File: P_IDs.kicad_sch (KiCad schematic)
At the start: 0 parts

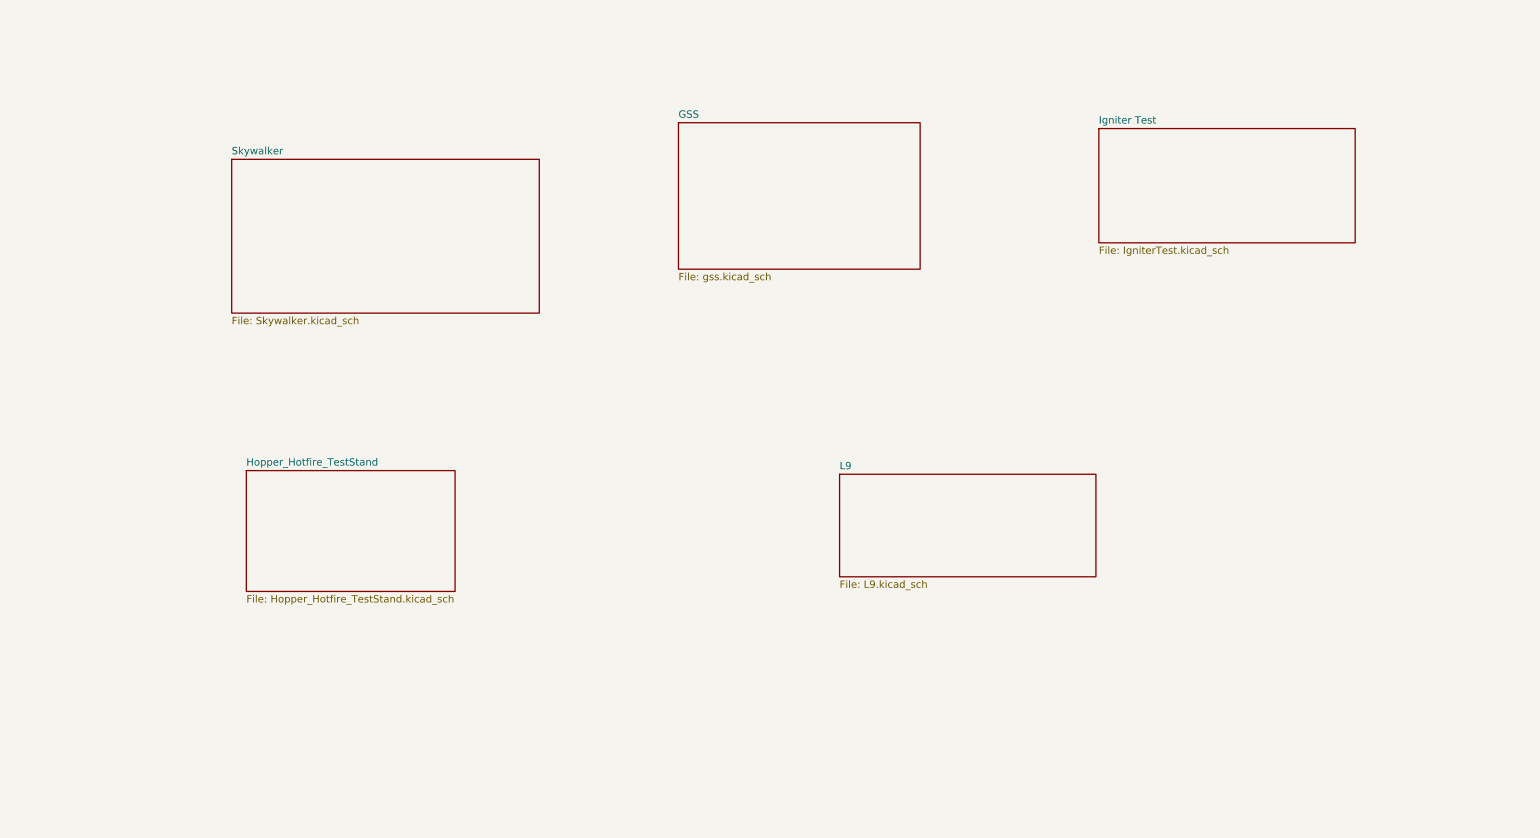
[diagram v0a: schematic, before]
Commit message: igniter+hotfire
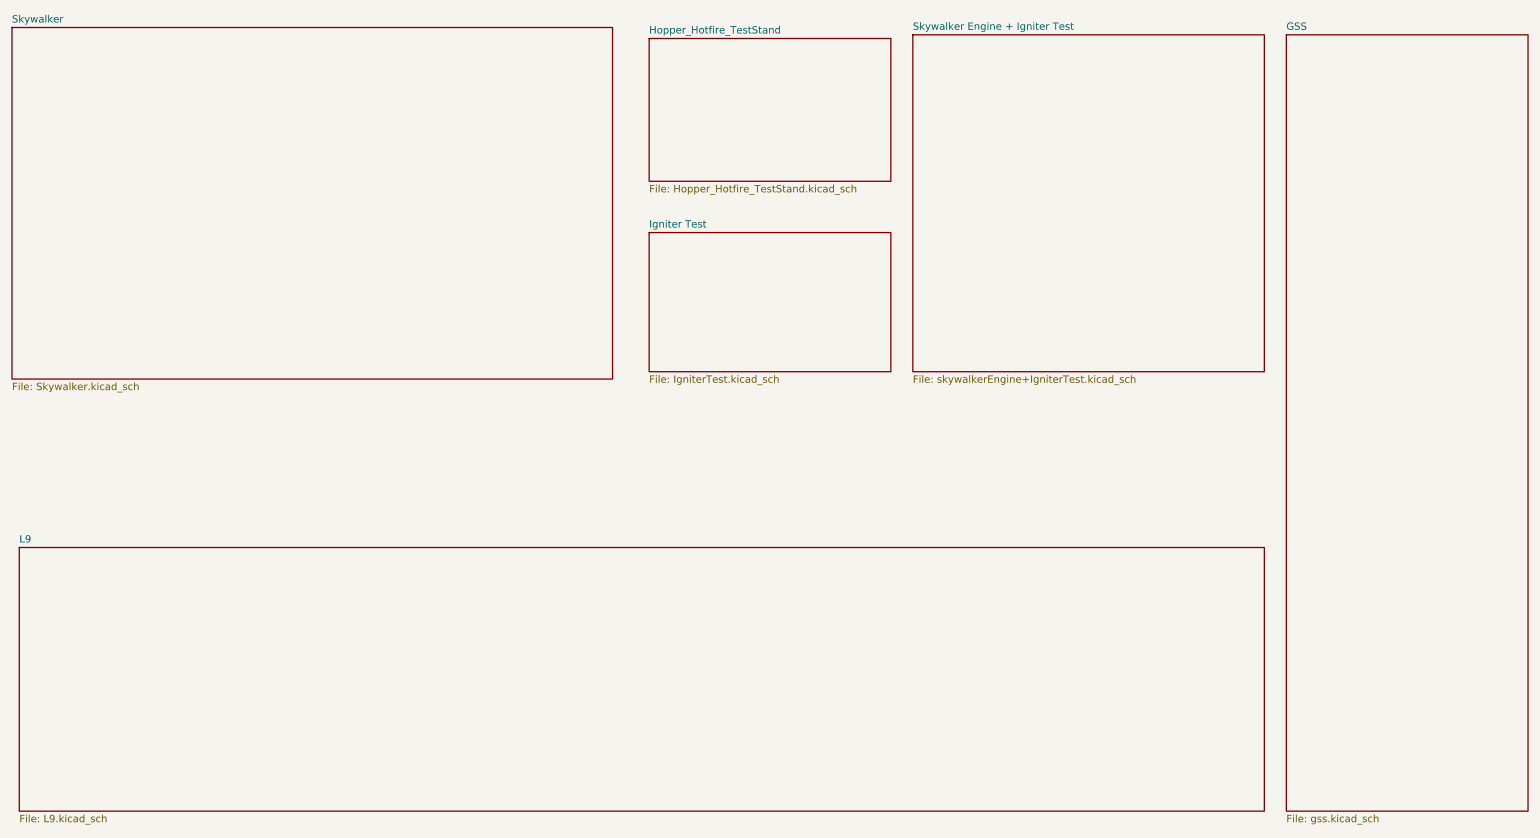
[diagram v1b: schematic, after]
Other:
- added sheet Skywalker Engine + Igniter Test (skywalkerEngine+IgniterTest.kicad_sch)
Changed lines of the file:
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@@
 	(paper "A4")
 	(sheet
-		(at 57.15 93.345)
-		(size 36.195 20.955)
+		(at 127 18.415)
+		(size 41.91 24.765)
 		(fields_autoplaced yes)
 		(stroke
@@
 		)
 		(property "Sheetname" "Hopper_Hotfire_TestStand"
-			(at 57.15 92.6334 0)
+			(at 127 17.7034 0)
 			(effects
 				(font
@@
 		)
 		(property "Sheetfile" "Hopper_Hotfire_TestStand.kicad_sch"
-			(at 57.15 114.8846 0)
+			(at 127 43.7646 0)
 			(effects
 				(font
@@
 	)
 	(sheet
-		(at 204.978 34.036)
-		(size 44.45 19.812)
+		(at 127 52.07)
+		(size 41.91 24.13)
 		(fields_autoplaced yes)
 		(stroke
@@
 		)
 		(property "Sheetname" "Igniter Test"
-			(at 204.978 33.3244 0)
+			(at 127 51.3584 0)
 			(effects
 				(font
@@
 		)
 		(property "Sheetfile" "IgniterTest.kicad_sch"
-			(at 204.978 54.4326 0)
+			(at 127 76.7846 0)
 			(effects
 				(font
@@
 	)
 	(sheet
-		(at 160.02 93.98)
-		(size 44.45 17.78)
+		(at 17.78 106.68)
+		(size 215.9 45.72)
 		(fields_autoplaced yes)
 		(stroke
@@
 		)
 		(property "Sheetname" "L9"
-			(at 160.02 93.2684 0)
+			(at 17.78 105.9684 0)
 			(effects
 				(font
@@
 		)
 		(property "Sheetfile" "L9.kicad_sch"
-			(at 160.02 112.3446 0)
+			(at 17.78 152.9846 0)
 			(effects
 				(font
@@
 	)
 	(sheet
-		(at 54.61 39.37)
-		(size 53.34 26.67)
+		(at 16.51 16.51)
+		(size 104.14 60.96)
 		(fields_autoplaced yes)
 		(stroke
@@
 		)
 		(property "Sheetname" "Skywalker"
-			(at 54.61 38.6584 0)
+			(at 16.51 15.7984 0)
 			(effects
 				(font
@@
 		)
 		(property "Sheetfile" "Skywalker.kicad_sch"
-			(at 54.61 66.6246 0)
+			(at 16.51 78.0546 0)
 			(effects
 				(font
@@
 		)
 		(property "Field2" ""
-			(at 54.61 39.37 0)
+			(at 16.51 16.51 0)
 			(effects
 				(font
@@
 	)
 	(sheet
-		(at 132.08 33.02)
-		(size 41.91 25.4)
+		(at 237.49 17.78)
+		(size 41.91 134.62)
 		(fields_autoplaced yes)
 		(stroke
@@
 		)
 		(property "Sheetname" "GSS"
-			(at 132.08 32.3084 0)
+			(at 237.49 17.0684 0)
 			(effects
 				(font
@@
 		)
 		(property "Sheetfile" "gss.kicad_sch"
-			(at 132.08 59.0046 0)
+			(at 237.49 152.9846 0)
 			(effects
 				(font
@@
 				)
 			)
+		)
+	)
+	(sheet
+		(at 172.72 17.78)
+		(size 60.96 58.42)
+		(fields_autoplaced yes)
+		(stroke
+			(width 0.1524)
+			(type solid)
+		)
+		(fill
+			(color 0 0 0 0.0000)
+		)
+		(property "Sheetname" "Skywalker Engine + Igniter Test"
+			(at 172.72 17.0684 0)
+			(effects
+				(font
+					(size 1.27 1.27)
+				)
+				(justify left bottom)
+			)
+		)
+		(property "Sheetfile" "skywalkerEngine+IgniterTest.kicad_sch"
+			(at 172.72 76.7846 0)
+			(effects
+				(font
+					(size 1.27 1.27)
+				)
+				(justify left top)
+			)
+		)
+		(instances
+			(project "P_IDs"
+				(path "/045f1f05-3134-4b6d-91b6-463031104f1e"
+					(page "7")
+				)
+			)
